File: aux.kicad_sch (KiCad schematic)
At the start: 19 parts, among them K601 EC2-12NU, M601 Fan_3pin, M602 Fan_3pin, Q601 2N7000, Q602 BC517, SW601 67F050, SW602 67F050

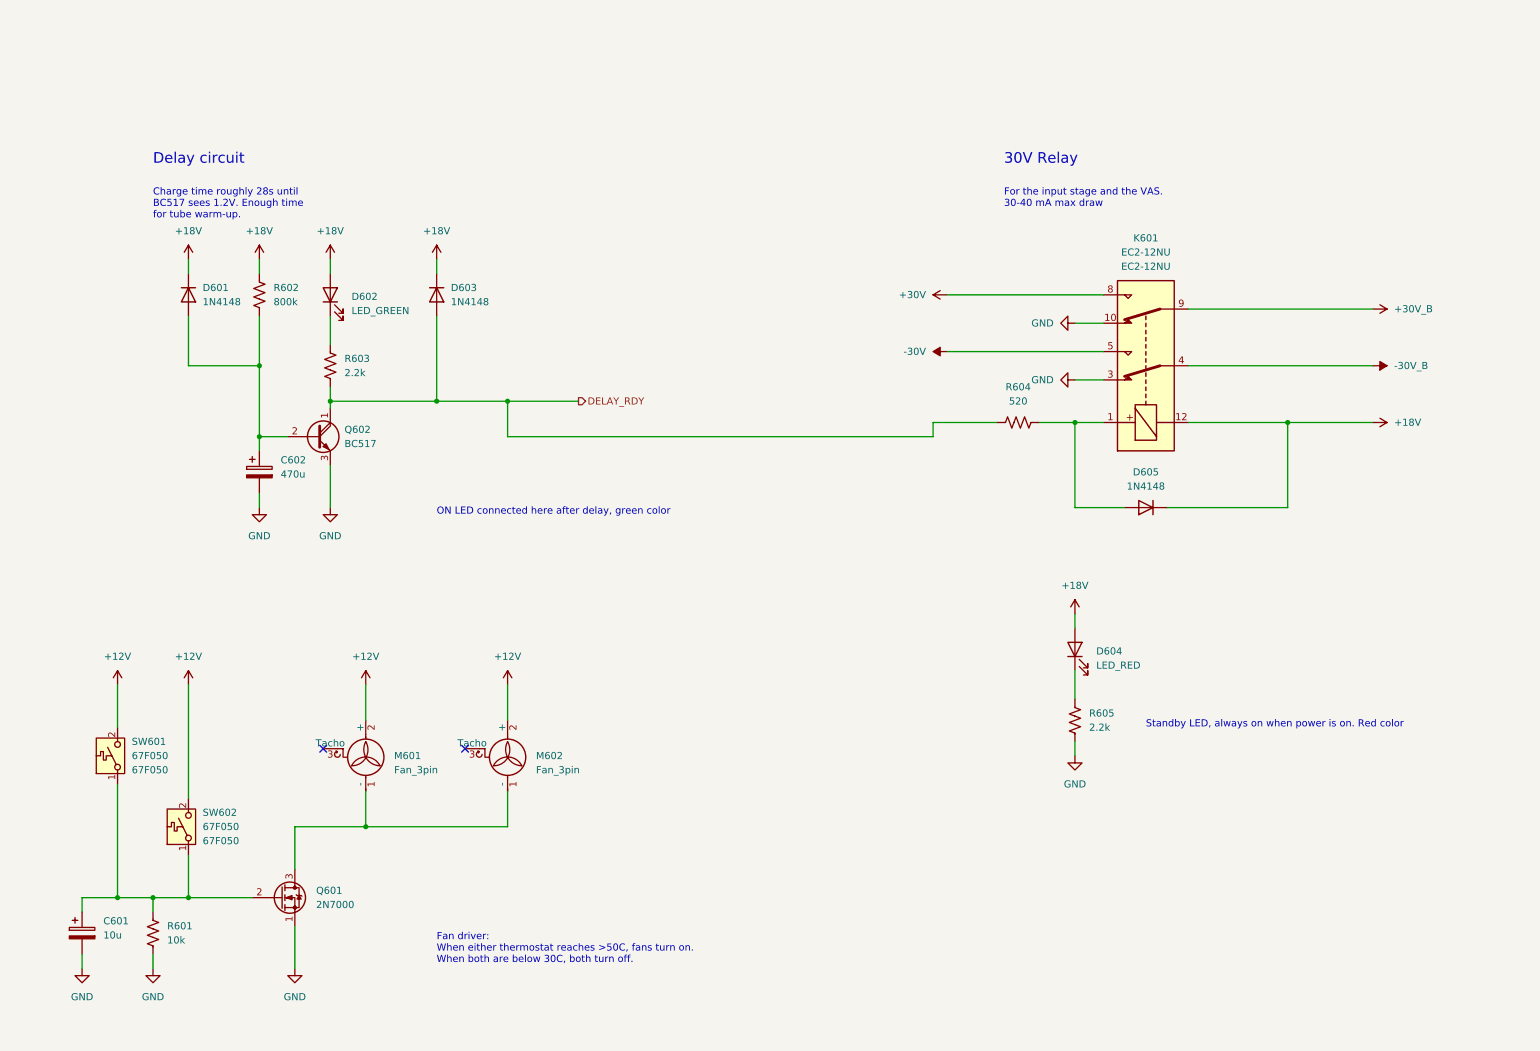
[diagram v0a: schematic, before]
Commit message: Completed schematic
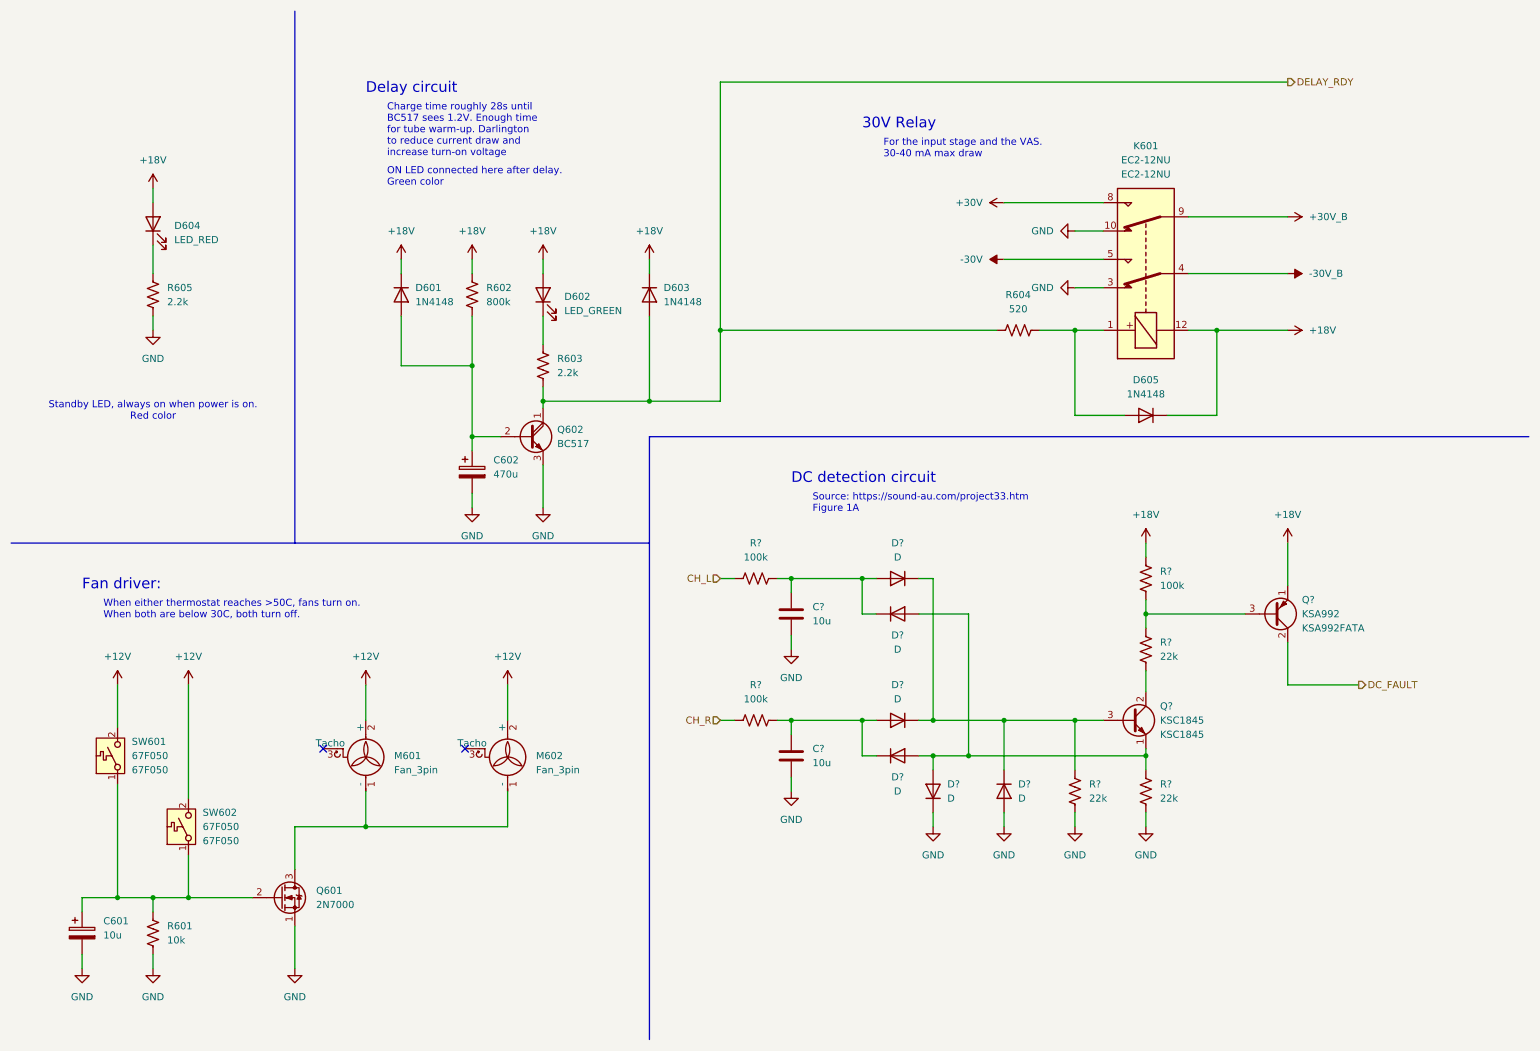
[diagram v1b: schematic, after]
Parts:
- added C? (x2): 10u, symbol Device:C
- added D? (x6): D, symbol Device:D
- added Q?: KSA992, symbol Transistor_BJT:Q_PNP_ECB
- added Q?: KSC1845, symbol Transistor_BJT:Q_NPN_ECB
- added R? (x3): 100k, symbol Device:R_US
- added R? (x3): 22k, symbol Device:R_US
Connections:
- net +18V: now also Q?.1 (E), R?.2
- net GND: now also C?.2, C?.2, D?.1 (K), D?.2 (A), R?.1, R?.1
- new net: Q?.3 (B), R?.1, R?.2
- new net: C?.1, D?.1 (K), D?.2 (A), R?.2 (x2)
- new net: D?.1 (K), D?.1 (K), D?.1 (K), Q?.3 (B), R?.2
- new net: Q?.2 (C), R?.1
- new net: D?.2 (A), D?.2 (A), D?.2 (A), Q?.1 (E), R?.2
- new net CH_L: R?.1
- new net CH_R: R?.1
- new net DC_FAULT: Q?.2 (C)
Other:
- note added: "Charge time roughly 28s until BC517 sees 1.2V. Enough time for tube warm-up. Darlington to reduce current draw and increase turn-on voltage"
- note added: "DC detection circuit"
- note added: "Fan driver:"
- note added: "ON LED connected here after delay. Green color"
- note added: "Source: https://sound-au.com/project33.htm Figure 1A"
- note added: "When either thermostat reaches >50C, fans turn on. When both are below 30C, both turn off."
- note removed: "Charge time roughly 28s until BC517 sees 1.2V. Enough time for tube warm-up."
- note removed: "Fan driver: When either thermostat reaches >50C, fans turn on. When both are below 30C, both turn off."
- note removed: "ON LED connected here after delay, green color"
- moved on the sheet: C602, D601, D602, D603, D604, D605, K601, Q602, R602, R603, R604, R605
